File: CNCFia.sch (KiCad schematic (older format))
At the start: 19 parts, among them J1 GND, J10 Driver_X, J11 Driver_Y, J12 Driver_Z, J14 Spin_10V, J15 Relay_1, J16 Relay_2, J17 Relay_3, J2 EXT_5V, J3 Limit SW_XY, J4 Limit SW_ZA, J5 Extra SW 0, J6 Extra SW 1, J7 EXT_12V, J8 OPTO_5V, J9 Signal Input

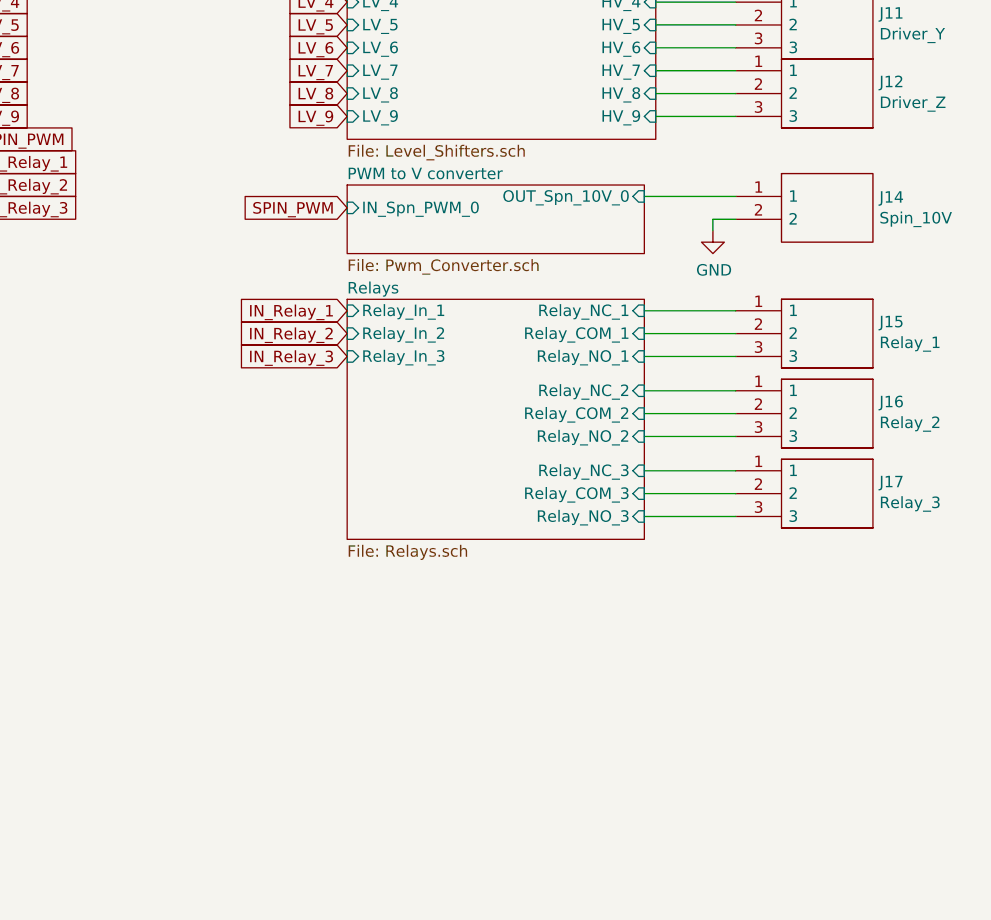
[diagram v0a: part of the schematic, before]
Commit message: Renamed Kicad Project, cleanup
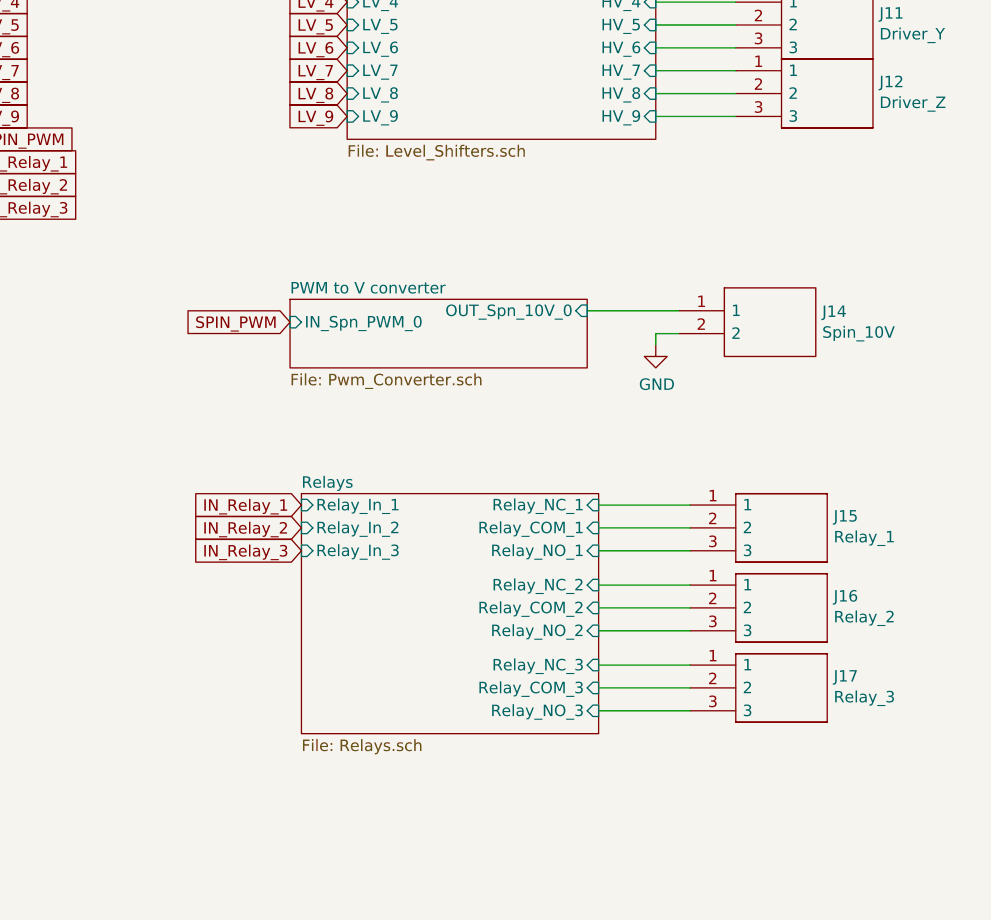
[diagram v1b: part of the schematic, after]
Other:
- moved on the sheet: J14, J15, J16, J17
